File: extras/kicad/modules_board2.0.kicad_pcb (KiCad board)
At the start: 2 copper layers, 176 x 104.1 mm, 12 parts

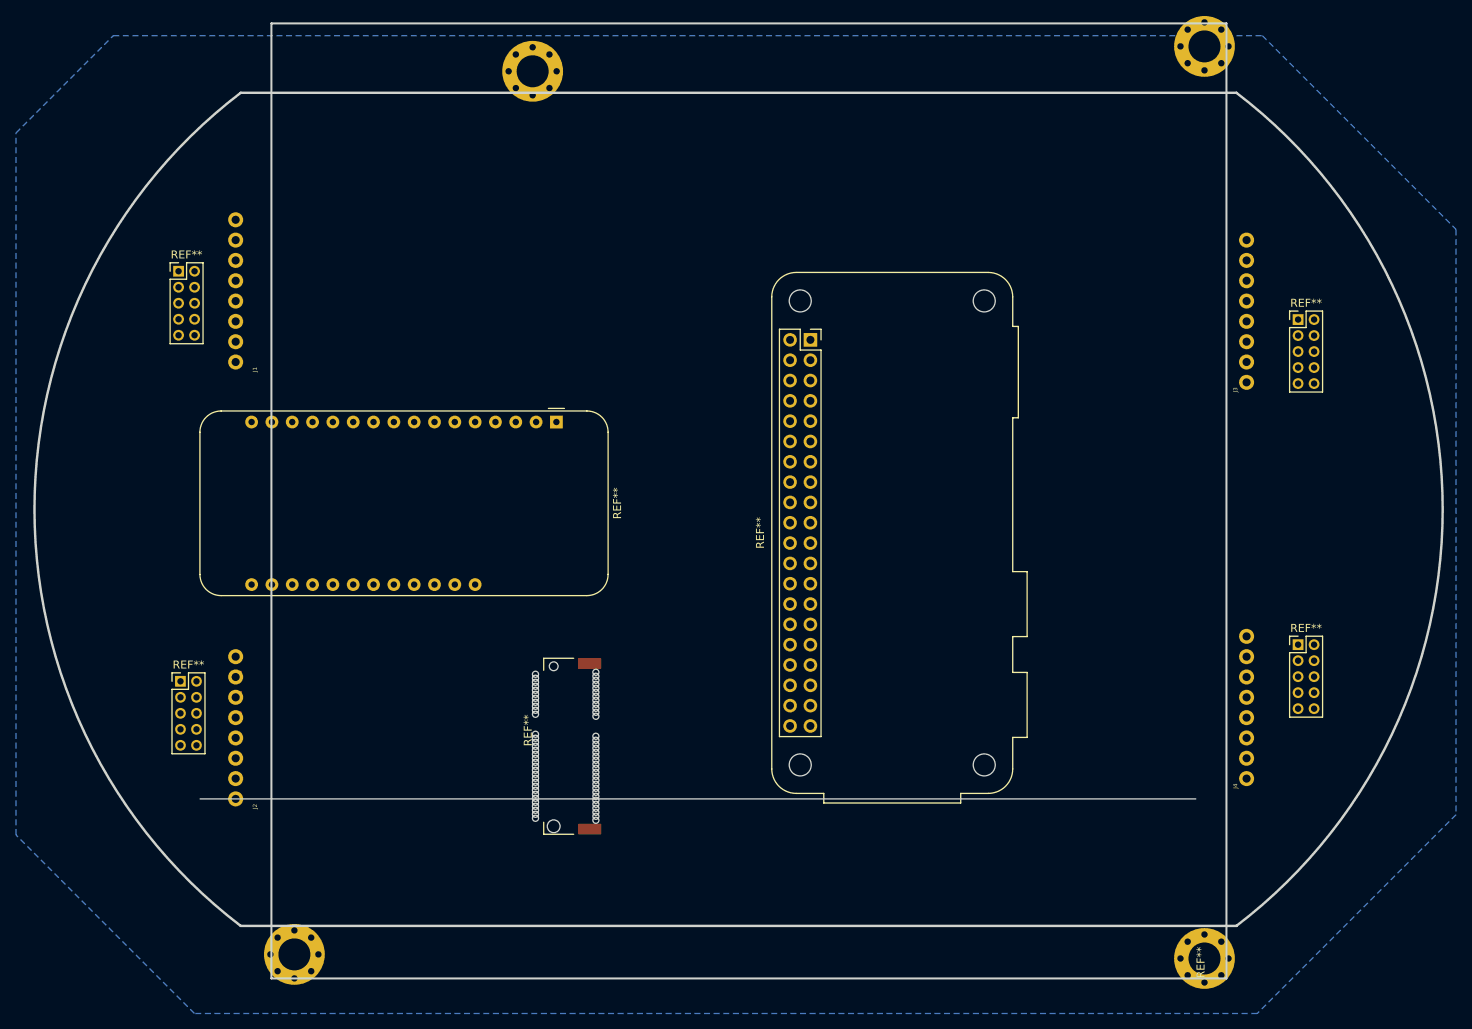
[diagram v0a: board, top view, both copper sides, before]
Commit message: Add files via upload
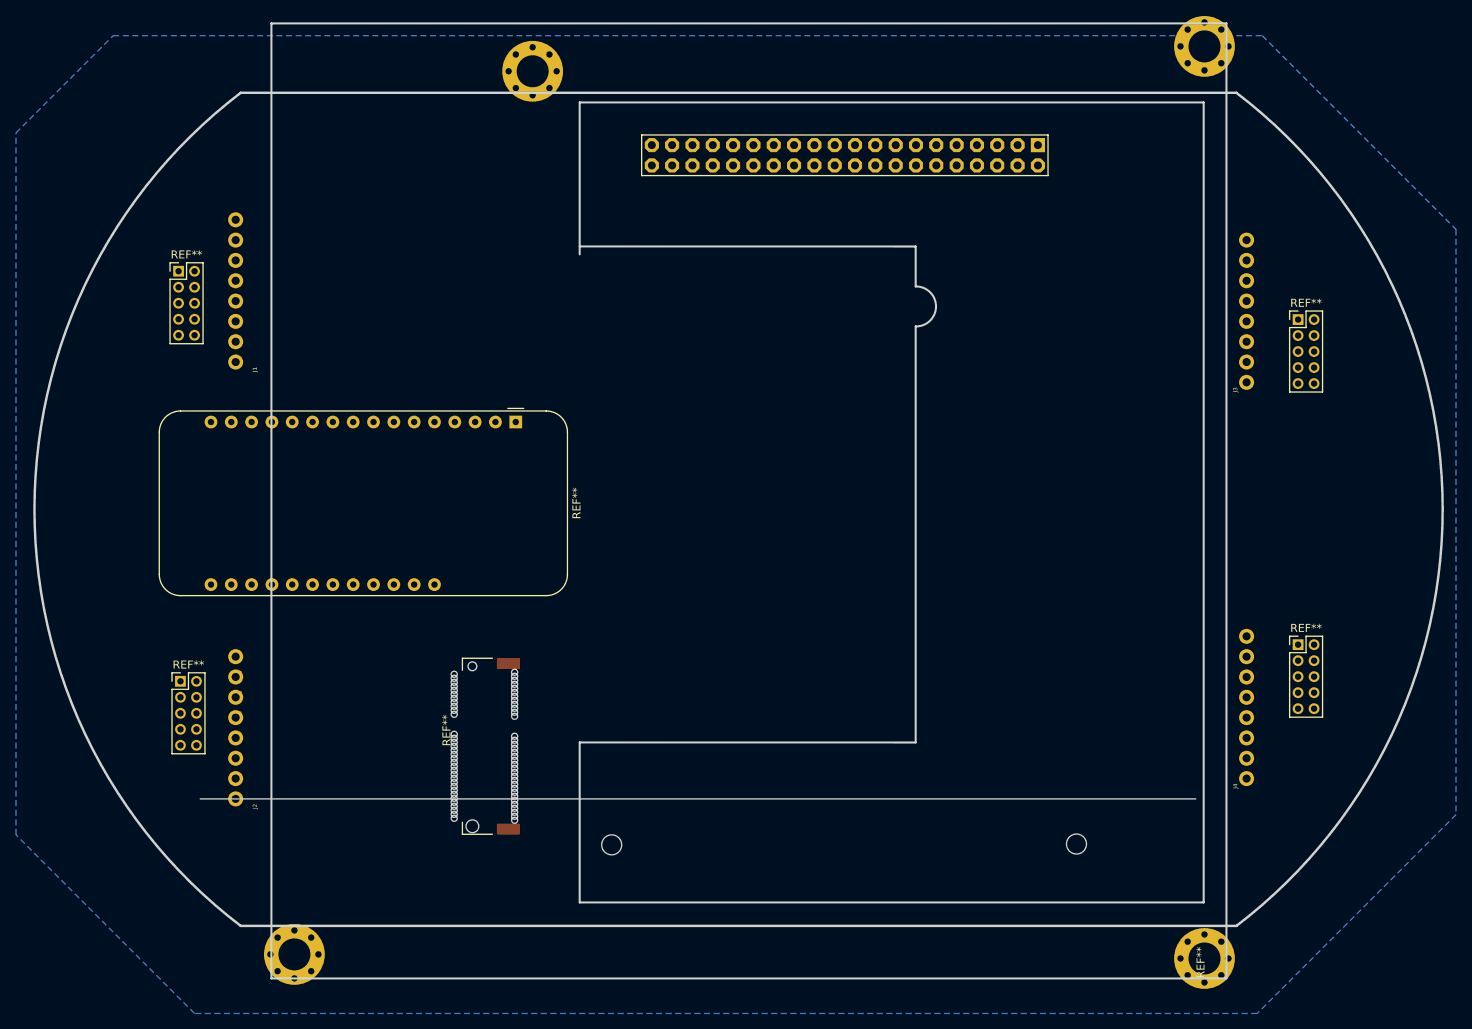
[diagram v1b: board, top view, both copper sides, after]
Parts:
- removed the REF** at (157.5, 83.8)
- added ?: , clipboard:cf6b2664-2037-41b6-b158-7ee893610716, F.Cu at (190.7, 146.8)
- moved REF** 10.2 mm to (115.2, 134.6)
- moved REF** 5.08 mm to (120.7, 94.1)

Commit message: Add files via upload
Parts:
- ?: footprint clipboard:cf6b2664-2037-41b6-b158-7ee893610716 -> Battery:cf6b2664-2037-41b6-b158-7ee893610716
- J1, J2, J3, J4: footprint 1X08_NO_SILK -> Battery:1X08_NO_SILK
- REF** (x4): footprint Connector_PinHeader_2.00mm:PinHeader_2x05_P2.00mm_Vertical -> Battery:PinHeader_2x05_P2.00mm_Vertical
- REF**: footprint Module:Adafruit_Feather -> Battery:Adafruit_Feather
- REF**: footprint Library:NANO-ITX_120X120 -> Battery:NANO-ITX_120X120
- REF**: footprint M.2-CONNECTOR-E -> Battery:M.2-CONNECTOR-E
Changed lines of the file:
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@@
   (net 13 "MOTOR_R_EN")
   (net 14 "BAT_GND")
-  (footprint "Connector_PinHeader_2.00mm:PinHeader_2x05_P2.00mm_Vertical" (layer "F.Cu")
+  (footprint "Battery:PinHeader_2x05_P2.00mm_Vertical" (layer "F.Cu")
     (at 78.74 126.5)
     (descr "Through hole straight pin header, 2x05, 2.00mm pitch, double rows")
@@
     )
   )
-  (footprint "1X08_NO_SILK" (layer "F.Cu")
+  (footprint "Battery:1X08_NO_SILK" (layer "F.Cu")
     (at 212.0011 138.6586 90)
     (descr "<h3>Plated Through Hole -8 Pin No Silk</h3>\n<p>Specifications:\n<ul><li>Pin count:8</li>\n<li>Pin pitch:0.1\"</li>\n</ul></p>\n<p>Example device(s):\n<ul><li>CONN_08</li>\n</ul></p>")
@@
       (net 3 "GND") (solder_mask_margin 0.0508))
   )
-  (footprint "Module:Adafruit_Feather" (layer "F.Cu")
+  (footprint "Battery:Adafruit_Feather" (layer "F.Cu")
     (at 120.65 94.0875 -90)
     (descr "Common footprint for the Adafruit Feather series of boards, https://learn.adafruit.com/adafruit-feather/feather-specification")
@@
     )
   )
-  (footprint "Library:NANO-ITX_120X120" (layer "F.Cu")
+  (footprint "Battery:NANO-ITX_120X120" (layer "F.Cu")
     (at 209.486 163.641 90)
     (attr through_hole)
@@
     (pad "P$45" thru_hole circle (at 111.296 -88.826 90) (size 1.308 1.308) (drill oval 0.8) (layers *.Cu *.Mask))
   )
-  (footprint "1X08_NO_SILK" (layer "F.Cu")
+  (footprint "Battery:1X08_NO_SILK" (layer "F.Cu")
     (at 212.0011 89.1286 90)
     (descr "<h3>Plated Through Hole -8 Pin No Silk</h3>\n<p>Specifications:\n<ul><li>Pin count:8</li>\n<li>Pin pitch:0.1\"</li>\n</ul></p>\n<p>Example device(s):\n<ul><li>CONN_08</li>\n</ul></p>")
@@
       (solder_mask_margin 0.0508))
   )
-  (footprint "M.2-CONNECTOR-E" (layer "F.Cu")
+  (footprint "Battery:M.2-CONNECTOR-E" (layer "F.Cu")
     (at 115.23 134.62 90)
     (attr through_hole)
@@
       ))
   )
-  (footprint "clipboard:cf6b2664-2037-41b6-b158-7ee893610716" (layer "F.Cu")
+  (footprint "Battery:cf6b2664-2037-41b6-b158-7ee893610716" (layer "F.Cu")
     (at 190.74 146.84)
     (fp_text reference "" (at 0 0) (layer "F.SilkS")
@@
       ))
   )
-  (footprint "1X08_NO_SILK" (layer "F.Cu")
+  (footprint "Battery:1X08_NO_SILK" (layer "F.Cu")
     (at 85.6361 86.5886 90)
     (descr "<h3>Plated Through Hole -8 Pin No Silk</h3>\n<p>Specifications:\n<ul><li>Pin count:8</li>\n<li>Pin pitch:0.1\"</li>\n</ul></p>\n<p>Example device(s):\n<ul><li>CONN_08</li>\n</ul></p>")
@@
       (solder_mask_margin 0.0508))
   )
-  (footprint "Connector_PinHeader_2.00mm:PinHeader_2x05_P2.00mm_Vertical" (layer "F.Cu")
+  (footprint "Battery:PinHeader_2x05_P2.00mm_Vertical" (layer "F.Cu")
     (at 78.5 75.24)
     (descr "Through hole straight pin header, 2x05, 2.00mm pitch, double rows")
@@
     )
   )
-  (footprint "1X08_NO_SILK" (layer "F.Cu")
+  (footprint "Battery:1X08_NO_SILK" (layer "F.Cu")
     (at 85.6361 141.1986 90)
     (descr "<h3>Plated Through Hole -8 Pin No Silk</h3>\n<p>Specifications:\n<ul><li>Pin count:8</li>\n<li>Pin pitch:0.1\"</li>\n</ul></p>\n<p>Example device(s):\n<ul><li>CONN_08</li>\n</ul></p>")
@@
       (net 3 "GND") (solder_mask_margin 0.0508))
   )
-  (footprint "Connector_PinHeader_2.00mm:PinHeader_2x05_P2.00mm_Vertical" (layer "F.Cu")
+  (footprint "Battery:PinHeader_2x05_P2.00mm_Vertical" (layer "F.Cu")
     (at 218.44 81.28)
     (descr "Through hole straight pin header, 2x05, 2.00mm pitch, double rows")
@@
     )
   )
-  (footprint "Connector_PinHeader_2.00mm:PinHeader_2x05_P2.00mm_Vertical" (layer "F.Cu")
+  (footprint "Battery:PinHeader_2x05_P2.00mm_Vertical" (layer "F.Cu")
     (at 218.44 121.92)
     (descr "Through hole straight pin header, 2x05, 2.00mm pitch, double rows")
